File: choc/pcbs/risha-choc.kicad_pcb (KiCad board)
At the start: 2 copper layers, 100 x 78.2 mm, 19 parts

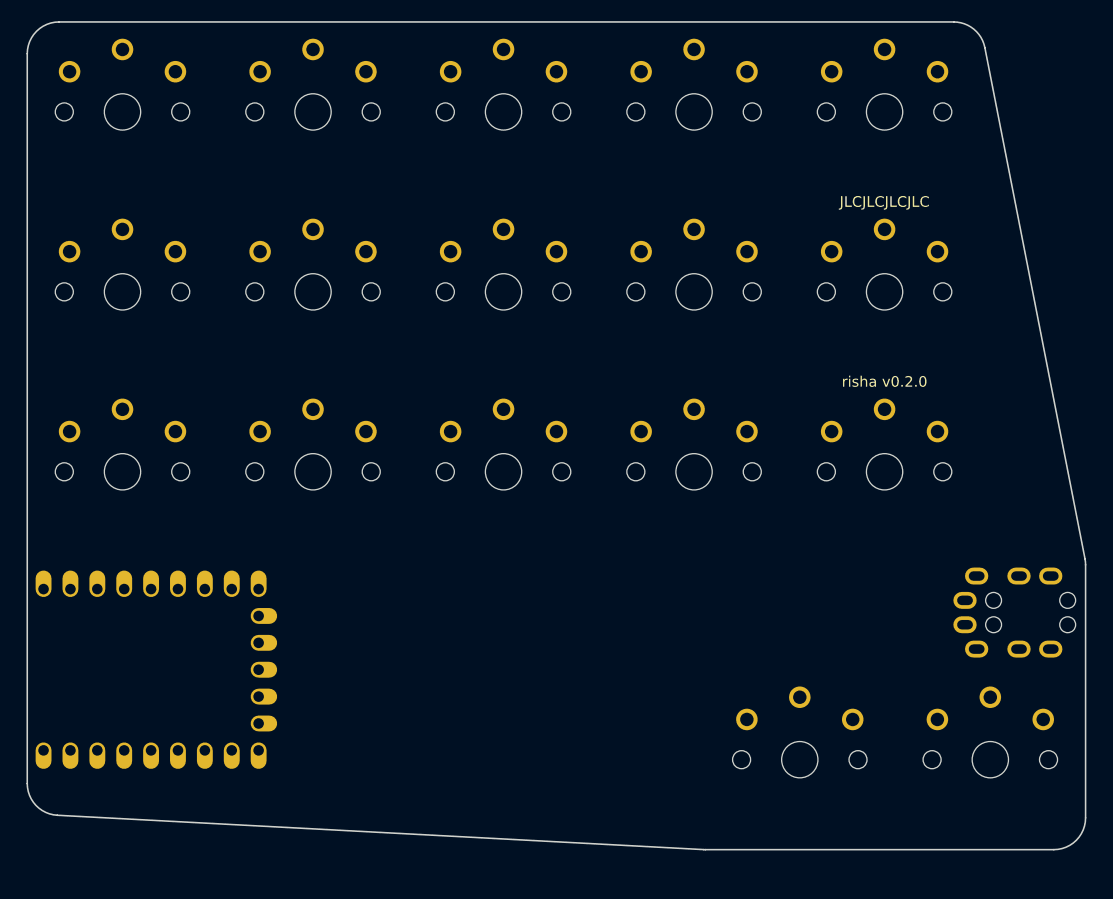
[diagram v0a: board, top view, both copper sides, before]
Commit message: hacky sub 100mm^2 idea for rear-facing trrs
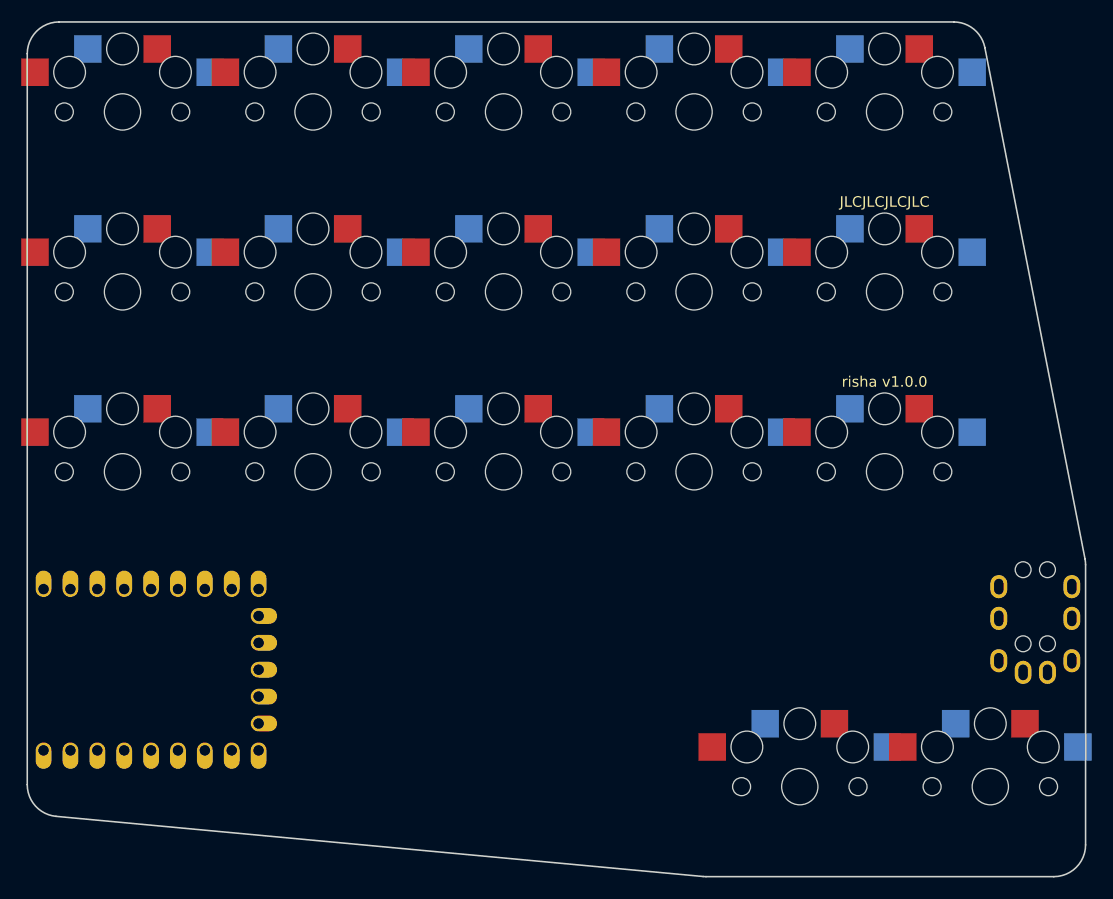
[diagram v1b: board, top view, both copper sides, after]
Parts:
- moved TRRS1 7.65 mm to (231.4, 143.7), turned to 0 degrees
- moved S16 2.55 mm to (208.0, 165.8)
- moved S17 2.55 mm to (226.0, 165.8)
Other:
- board size 100 x 78.2 mm -> 100 x 80.8 mm
- board text added: "risha v1.0.0"
- board text removed: "risha v0.2.0"

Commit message: trying new choc outline
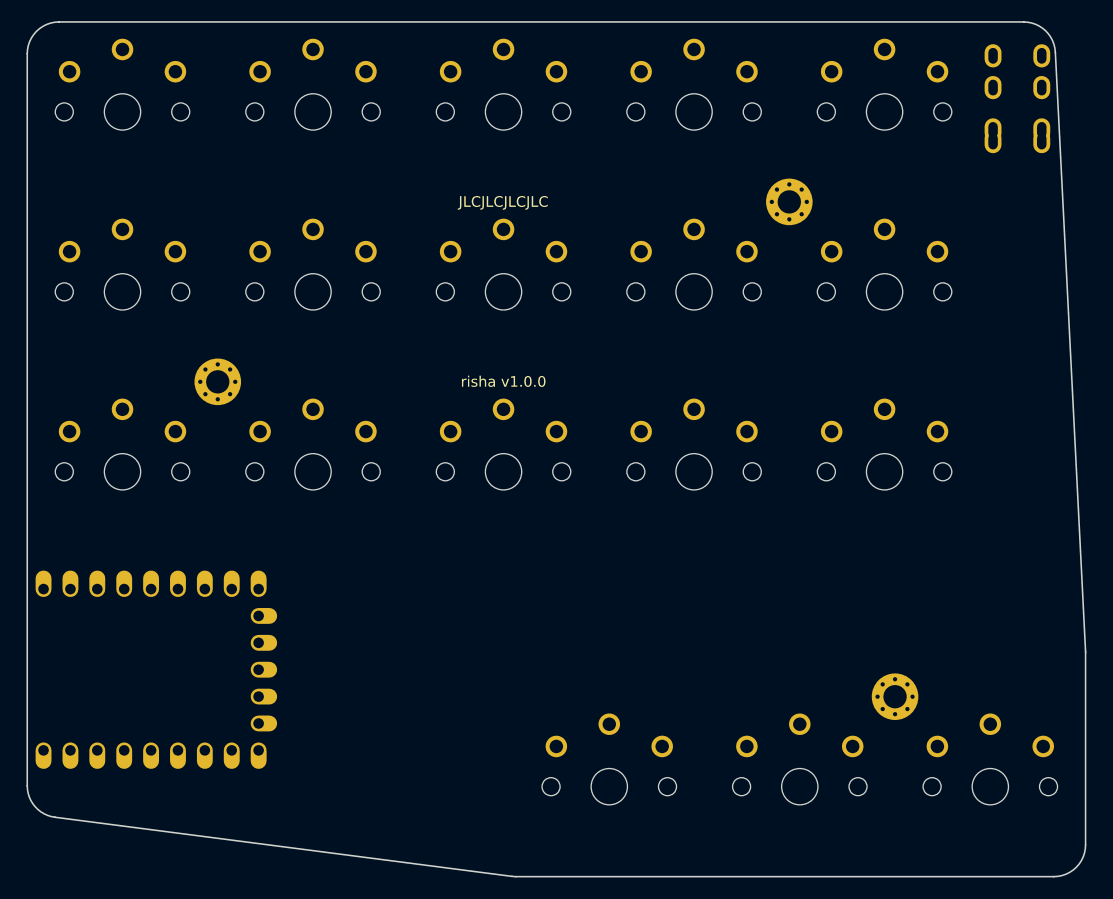
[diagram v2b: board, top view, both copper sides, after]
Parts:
- added S18: , PG1350, F.Cu at (226.0, 165.8)
- added _4: , MountingHole_2.2mm_M2_Pad_Via, F.Cu at (153.0, 127.5)
- added _5: , MountingHole_2.2mm_M2_Pad_Via, F.Cu at (207.0, 110.5)
- added _6: , MountingHole_2.2mm_M2_Pad_Via, F.Cu at (217.0, 157.2)
- moved TRRS1 50.2 mm to (230.8, 93.5)
- moved S16 18.0 mm to (190.0, 165.8)
- moved S17 18.0 mm to (208.0, 165.8)
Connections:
- ? pad 10: GP9 -> matrix_index_bottom
- ? pad 11: matrix_middle_bottom -> matrix_index_home
- ? pad 13: matrix_index_home -> GP12
- ? pad 14: matrix_index_bottom -> matrix_inner_top
- ? pad 15: matrix_inner_bottom -> matrix_inner_home
- ? pad 16: matrix_inner_home -> matrix_inner_bottom
- ? pad 17: matrix_inner_top -> thumbfan_near_home
- ? pad 18: thumbfan_near_home -> thumbfan_home_home
- ? pad 9: GP8 -> matrix_middle_bottom
- S17 pad 1: thumbfan_far_home -> thumbfan_middle_home
- TRRS1 pad 1: 3V3 -> GND
- TRRS1 pad 3: GP9 -> VSYS
- TRRS1 pad 4: GP8 -> GP16
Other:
- outline, holes or cut-outs redrawn
